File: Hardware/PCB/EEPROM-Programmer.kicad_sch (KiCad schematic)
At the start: 21 parts, among them U10 74HC595, U11 74HC595, U12 74HC595, U13 MCP2221AxP, U2 74HC04, U9 74HC165

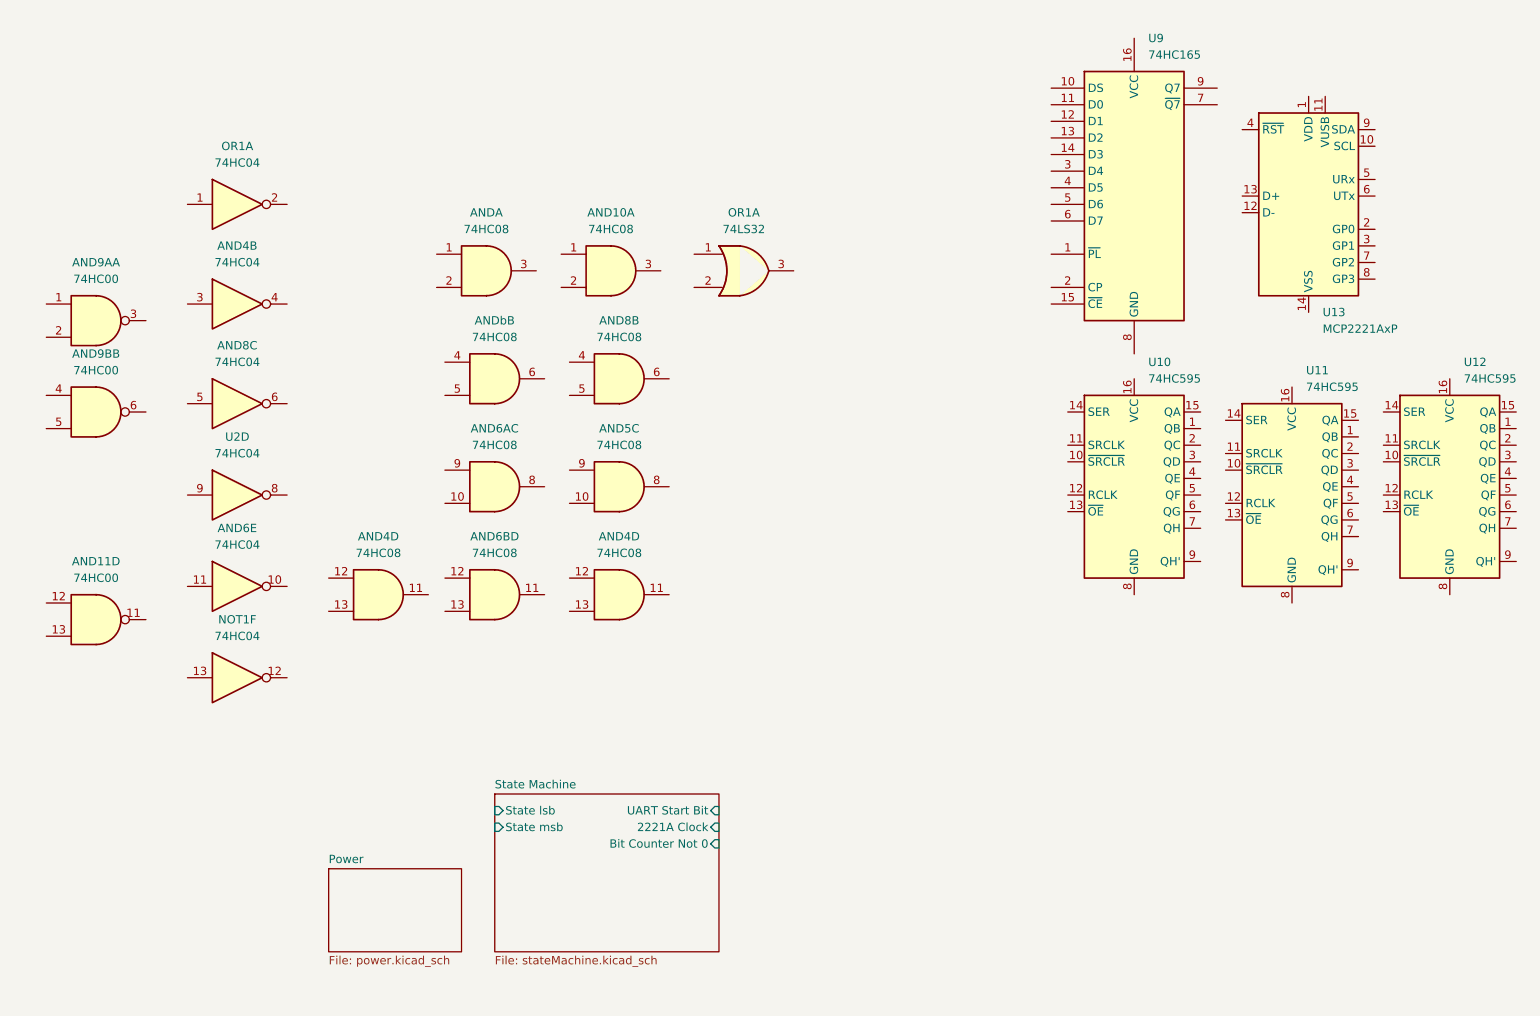
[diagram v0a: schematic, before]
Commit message: Writing maybe working, also started on other parts of schematic
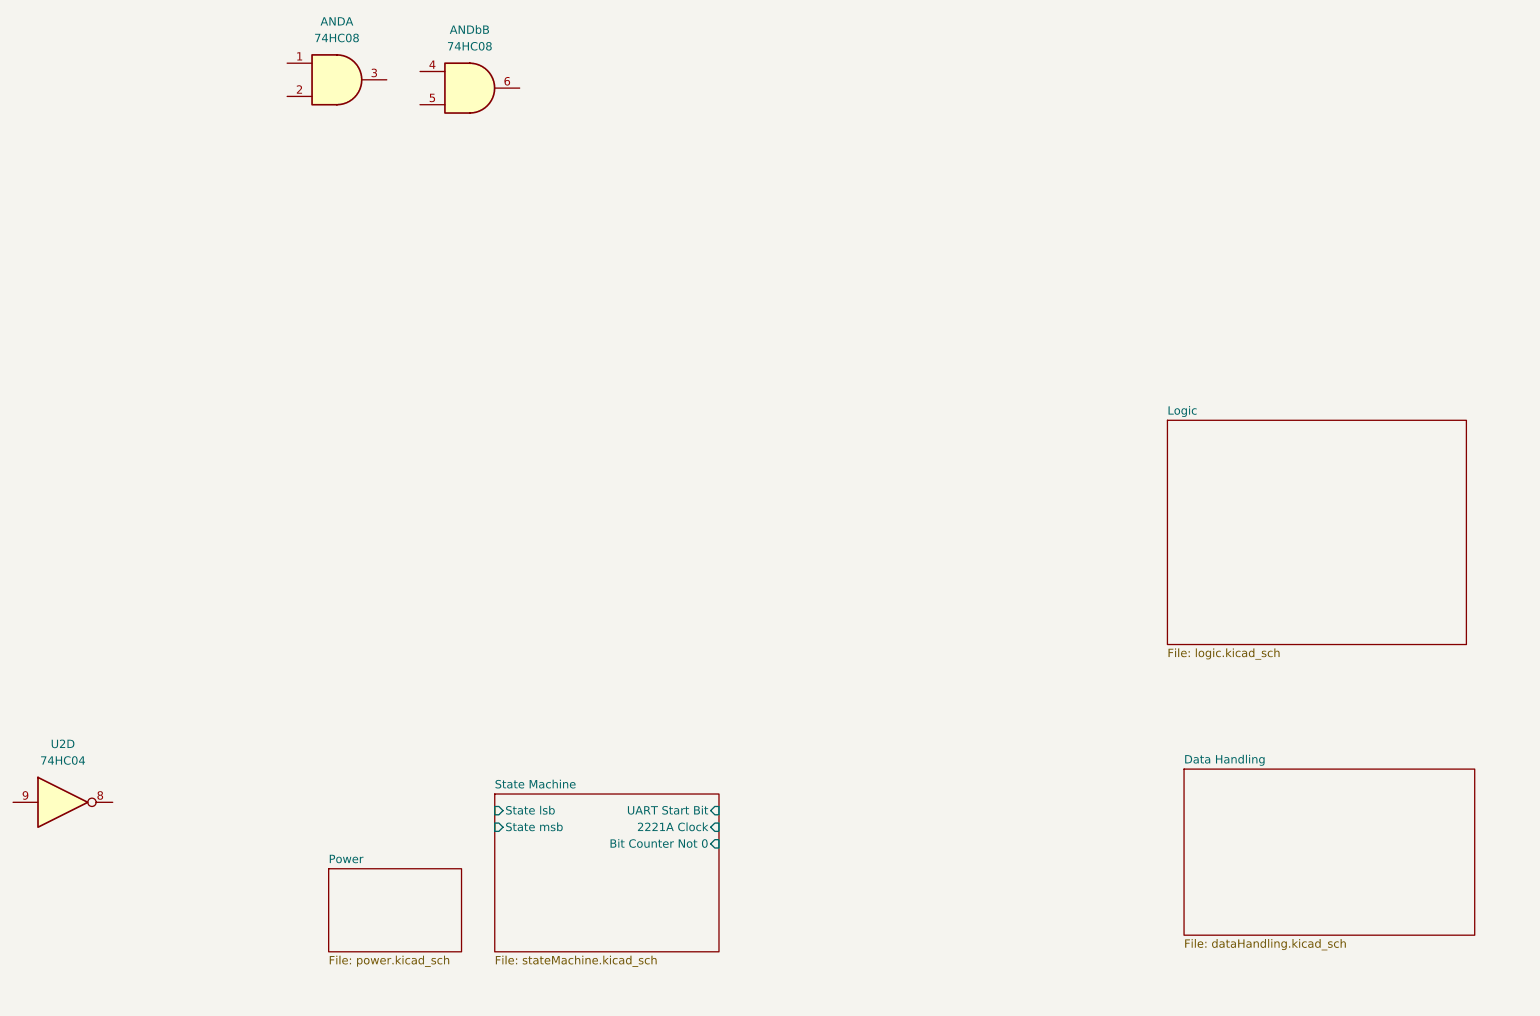
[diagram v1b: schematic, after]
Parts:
- removed AND10, AND4 (x2), AND5, AND6A, AND6B: 74HC08, symbol 74xx:74LS08
- removed AND11, AND9A, AND9B: 74HC00, Package_DIP:DIP-14_W7.62mm_Socket, symbol 74xx:74HC00
- removed AND6, AND8, NOT1, OR1: 74HC04, symbol 74xx:74HC04
- removed OR1: 74LS32, symbol 74xx:74LS32
- removed U10, U11, U12: 74HC595, symbol 74xx:74HC595
- removed U13: MCP2221AxP, Package_DIP:DIP-14_W7.62mm_Socket, symbol Interface_USB:MCP2221AxP
- removed U9: 74HC165, symbol 74xx:74HC165
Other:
- added sheet Data Handling (dataHandling.kicad_sch)
- added sheet Logic (logic.kicad_sch)
- moved on the sheet: ANDA, ANDbB, U2D

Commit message: Finished schematic
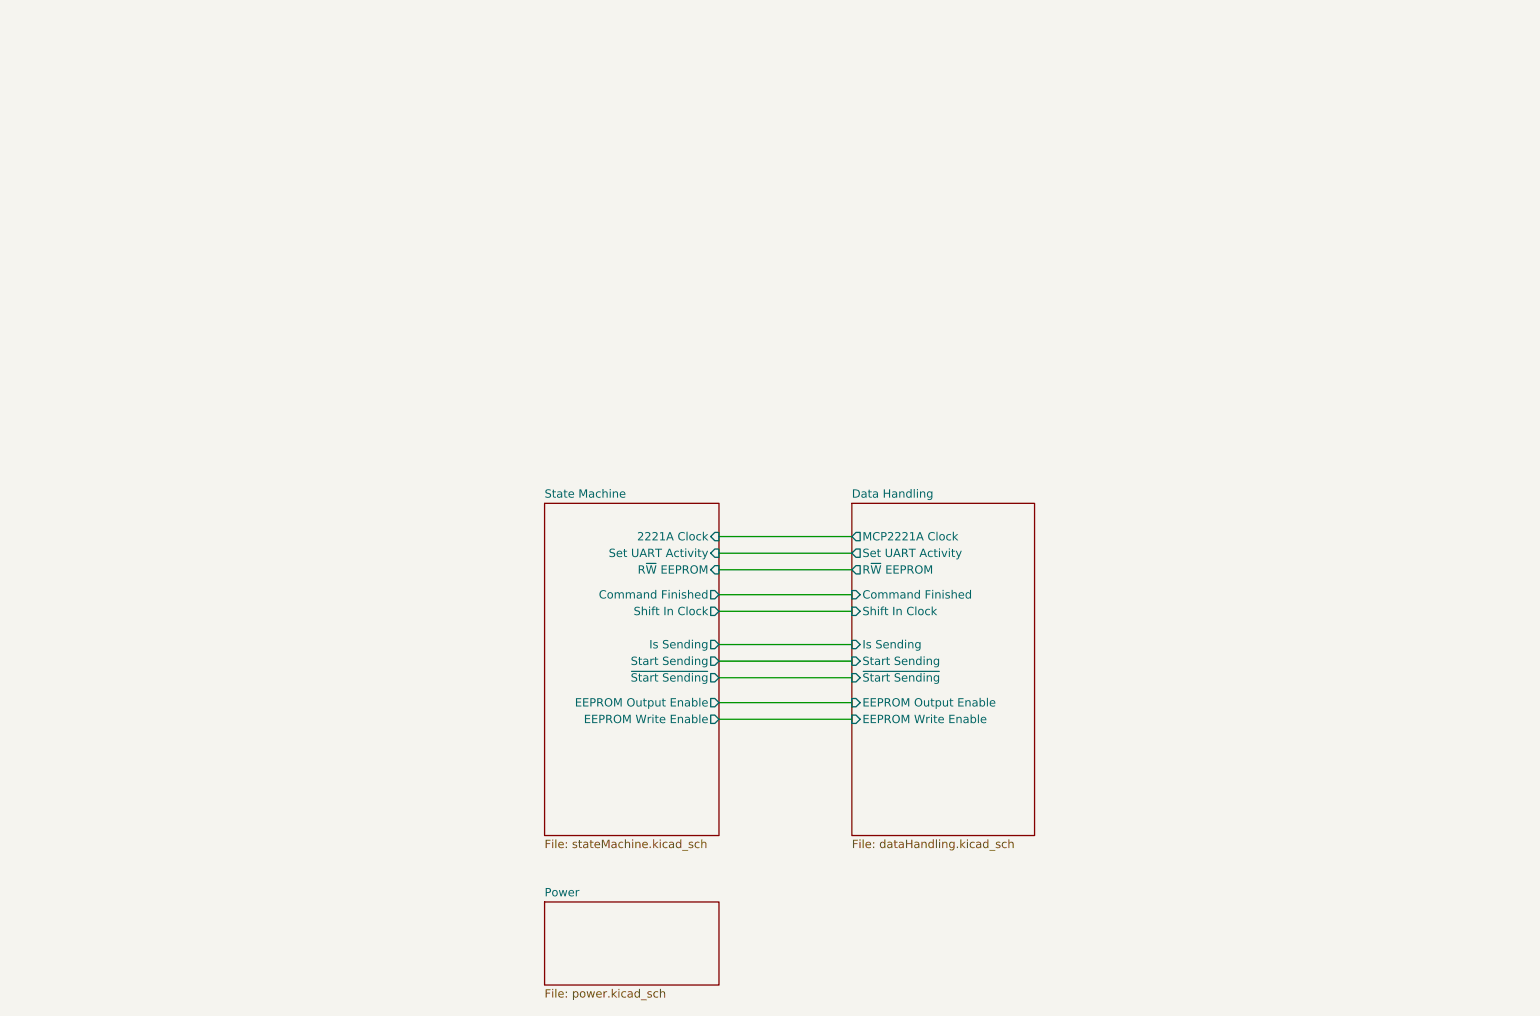
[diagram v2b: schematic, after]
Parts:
- removed AND, ANDb: 74HC08, symbol 74xx:74LS08
- removed U2: 74HC04, symbol 74xx:74HC04
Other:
- removed sheet Logic
- sheet Data Handling ports: added Command Finished, EEPROM Output Enable, EEPROM Write Enable, Is Sending, MCP2221A Clock, R~{W} EEPROM, Set UART Activity, Shift In Clock, Start Sending, ~{Start Sending}; removed none
- sheet State Machine ports: added Command Finished, EEPROM Output Enable, EEPROM Write Enable, Is Sending, R~{W} EEPROM, Set UART Activity, Shift In Clock, Start Sending, ~{Start Sending}; removed Bit Counter Not 0, State lsb, State msb, UART Start Bit
